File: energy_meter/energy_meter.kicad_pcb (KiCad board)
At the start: 2 copper layers, 123 parts, among them IC1 ADUM4151BRIZ, IC2 ADUM6404ARIZ, IC3 ADP122AUJZ-3.3-R7, J1 Screw_Terminal_01x02, J2 Screw_Terminal_01x02, T1 T60404-E4626-X502, T2 T60404-E4626-X502, U1 ADE9000ACPZ, U2 SN74LV4T125PWR, U3 SN74LV4T125PWR, Y1 Crystal_GND24

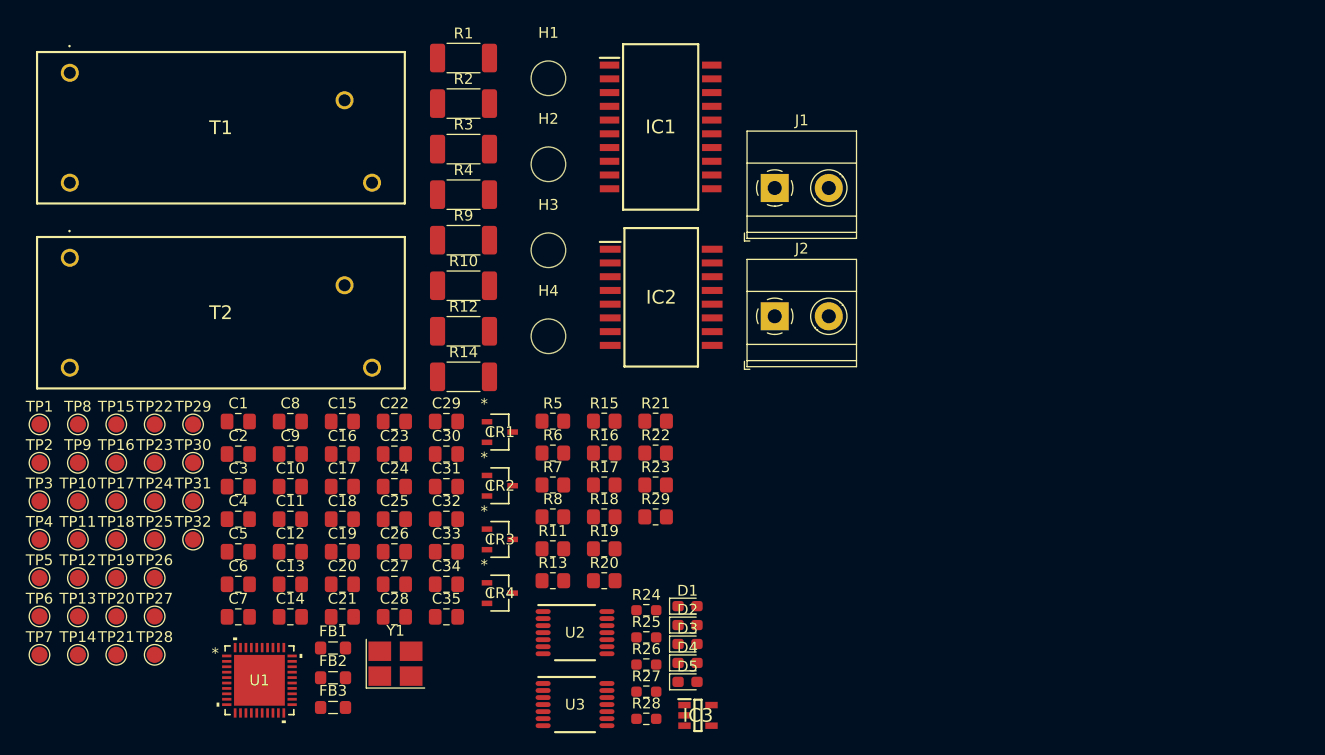
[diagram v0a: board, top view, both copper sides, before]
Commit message: Finish up schematic
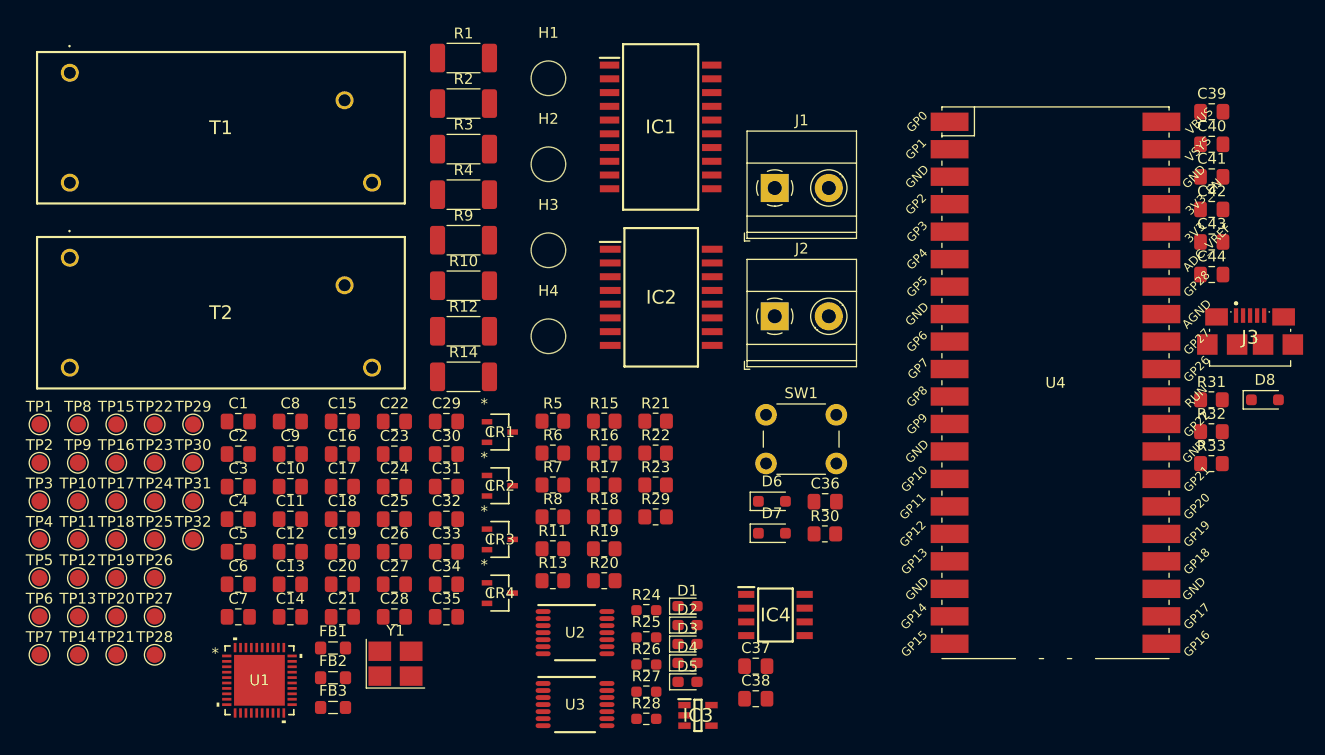
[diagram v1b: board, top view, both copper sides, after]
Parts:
- added C36: 1u, Capacitor_SMD:C_0805_2012Metric_Pad1.18x1.45mm_HandSolder, F.Cu at (100.6, 68.1)
- added C37: 4.7u, Capacitor_SMD:C_0805_2012Metric_Pad1.18x1.45mm_HandSolder, F.Cu at (94.2, 83.3)
- added C38: 0.1u, Capacitor_SMD:C_0805_2012Metric_Pad1.18x1.45mm_HandSolder, F.Cu at (94.2, 86.4)
- added C39: 0.1u, Capacitor_SMD:C_0805_2012Metric_Pad1.18x1.45mm_HandSolder, F.Cu at (136.4, 32.1)
- added C40: 10u, Capacitor_SMD:C_0805_2012Metric_Pad1.18x1.45mm_HandSolder, F.Cu at (136.4, 35.1)
- added C41: 0.1u, Capacitor_SMD:C_0805_2012Metric_Pad1.18x1.45mm_HandSolder, F.Cu at (136.4, 38.1)
- added C42: 10u, Capacitor_SMD:C_0805_2012Metric_Pad1.18x1.45mm_HandSolder, F.Cu at (136.4, 41.1)
- added C43: 22u, Capacitor_SMD:C_0805_2012Metric_Pad1.18x1.45mm_HandSolder, F.Cu at (136.4, 44.1)
- added C44: 0.1u, Capacitor_SMD:C_0805_2012Metric_Pad1.18x1.45mm_HandSolder, F.Cu at (136.4, 47.1)
- added D6: D_Schottky, Diode_SMD:D_SOD-323_HandSoldering, F.Cu at (95.7, 68.1)
- added D7: D_Schottky, Diode_SMD:D_SOD-323_HandSoldering, F.Cu at (95.7, 71.1)
- added D8: D_Schottky, Diode_SMD:D_SOD-323_HandSoldering, F.Cu at (141.3, 58.7)
- added IC4: 24LC32A_SN, 24LC32A_SN:SOIC127P600X175-8N, F.Cu at (96.0, 78.6)
- added J3: ZX62-AB-5PA_31_, microUSB:ZX62AB5PA31, F.Cu at (139.9, 53.0)
- added R30: 10k, Resistor_SMD:R_0805_2012Metric_Pad1.20x1.40mm_HandSolder, F.Cu at (100.6, 71.1)
- added R31: 10k, Resistor_SMD:R_0805_2012Metric_Pad1.20x1.40mm_HandSolder, F.Cu at (136.3, 58.7)
- added R32: 10k, Resistor_SMD:R_0805_2012Metric_Pad1.20x1.40mm_HandSolder, F.Cu at (136.3, 61.7)
- added R33: 10k, Resistor_SMD:R_0805_2012Metric_Pad1.20x1.40mm_HandSolder, F.Cu at (136.3, 64.6)
- added SW1: SW_Push, Button_Switch_THT:SW_PUSH_6mm, F.Cu at (95.2, 60.1)
- added U4: Pico_SMD_NODEBUG, RPi Pico:RPi_PicoW_SMD, F.Cu at (121.9, 57.1)
